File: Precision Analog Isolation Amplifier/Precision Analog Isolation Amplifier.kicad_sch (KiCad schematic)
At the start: 58 parts, among them IC1 ADA4899-1YRDZ, J1 Conn_01x03, J2 Conn_01x03, J3 Conn_Coaxial, J4 Conn_Coaxial, Q1 ---, U1 HCNR201, U2 ADA4522, U4 ADA4522

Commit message: update pcb
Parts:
- J3, J4: footprint Connector_Coaxial:SMA_Amphenol_132289_EdgeMount -> CONN SMA JACK STR 50 OHM SMD:CONN_732511350_MOL
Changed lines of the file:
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@@
 			)
 		)
-		(property "Footprint" "Connector_Coaxial:SMA_Amphenol_132289_EdgeMount"
+		(property "Footprint" "CONN SMA JACK STR 50 OHM SMD:CONN_732511350_MOL"
 			(at 38.1 66.04 0)
 			(effects
@@
 			)
 		)
-		(property "Footprint" "Connector_Coaxial:SMA_Amphenol_132289_EdgeMount"
+		(property "Footprint" "CONN SMA JACK STR 50 OHM SMD:CONN_732511350_MOL"
 			(at 262.89 43.18 0)
 			(effects

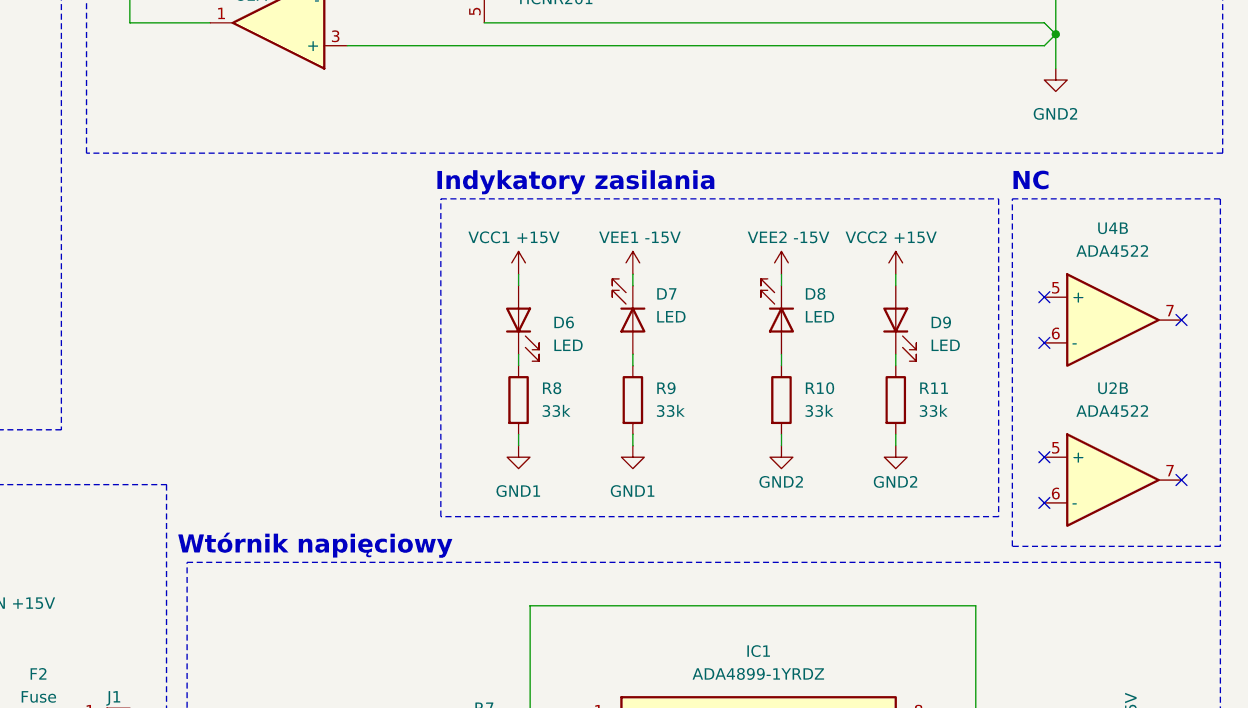
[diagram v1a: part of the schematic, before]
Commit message: Update PCB & Schematic
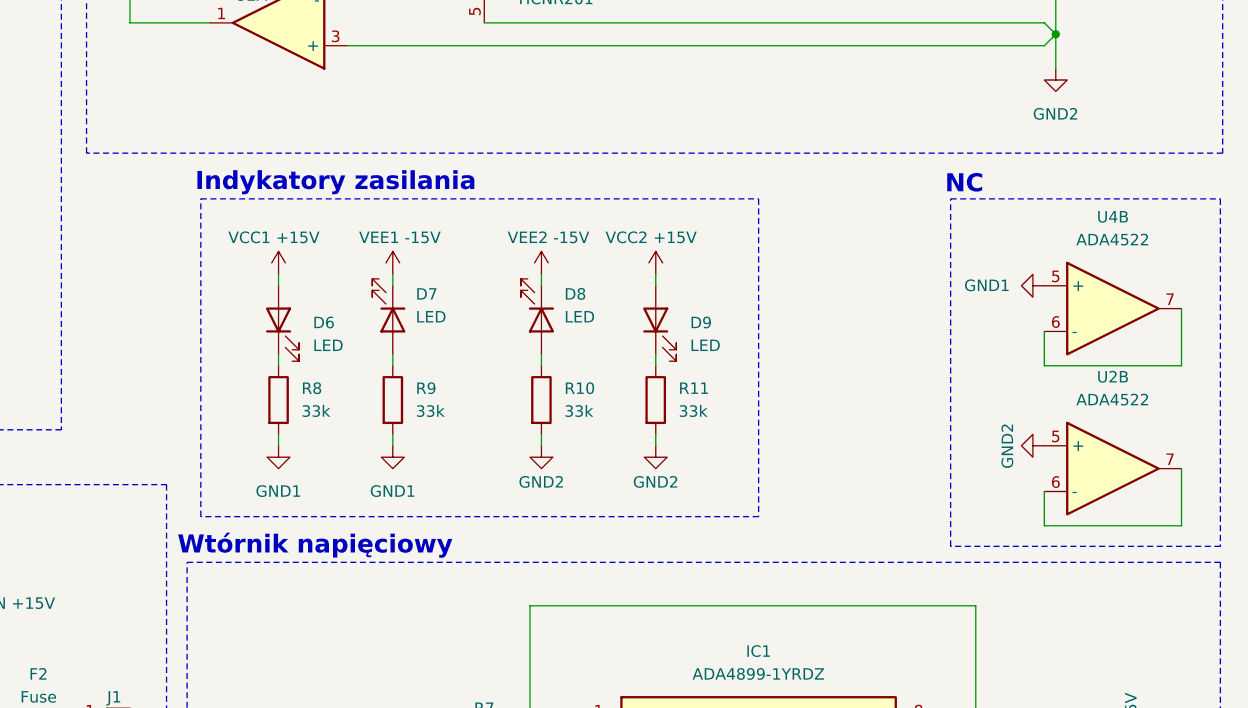
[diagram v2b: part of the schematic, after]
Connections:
- net GND1: now also U4.5 (+)
- net GND2: now also U2.5 (+)
- net at U4.6 (-): now also U4.7
- net at U2.6 (-): now also U2.7
- no-connect marks 9 -> 3
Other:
- moved on the sheet: D6, D7, D8, D9, R10, R11, R8, R9, U2B, U4B
